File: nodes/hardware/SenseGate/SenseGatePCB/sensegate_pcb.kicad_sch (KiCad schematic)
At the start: 25 parts, among them J1 Conn_01x02_Pin, J10 Conn_01x02_Pin, J11 Conn_01x02_Pin, J2 Conn_01x02_Socket, J3 Conn_01x02_Socket, J4 Conn_01x24_Pin, J5 Conn_01x04_Socket, J6 Conn_01x04_Socket, J7 Conn_01x04_Socket, J8 Conn_01x04_Socket, J9 Conn_01x02_Socket, Q4 SS8050, SW1 SW_Reed, SW2 SW_Reed, SW3 SW_Reed, SW5 SW_DPDT_x2, U1 DD05CVSA

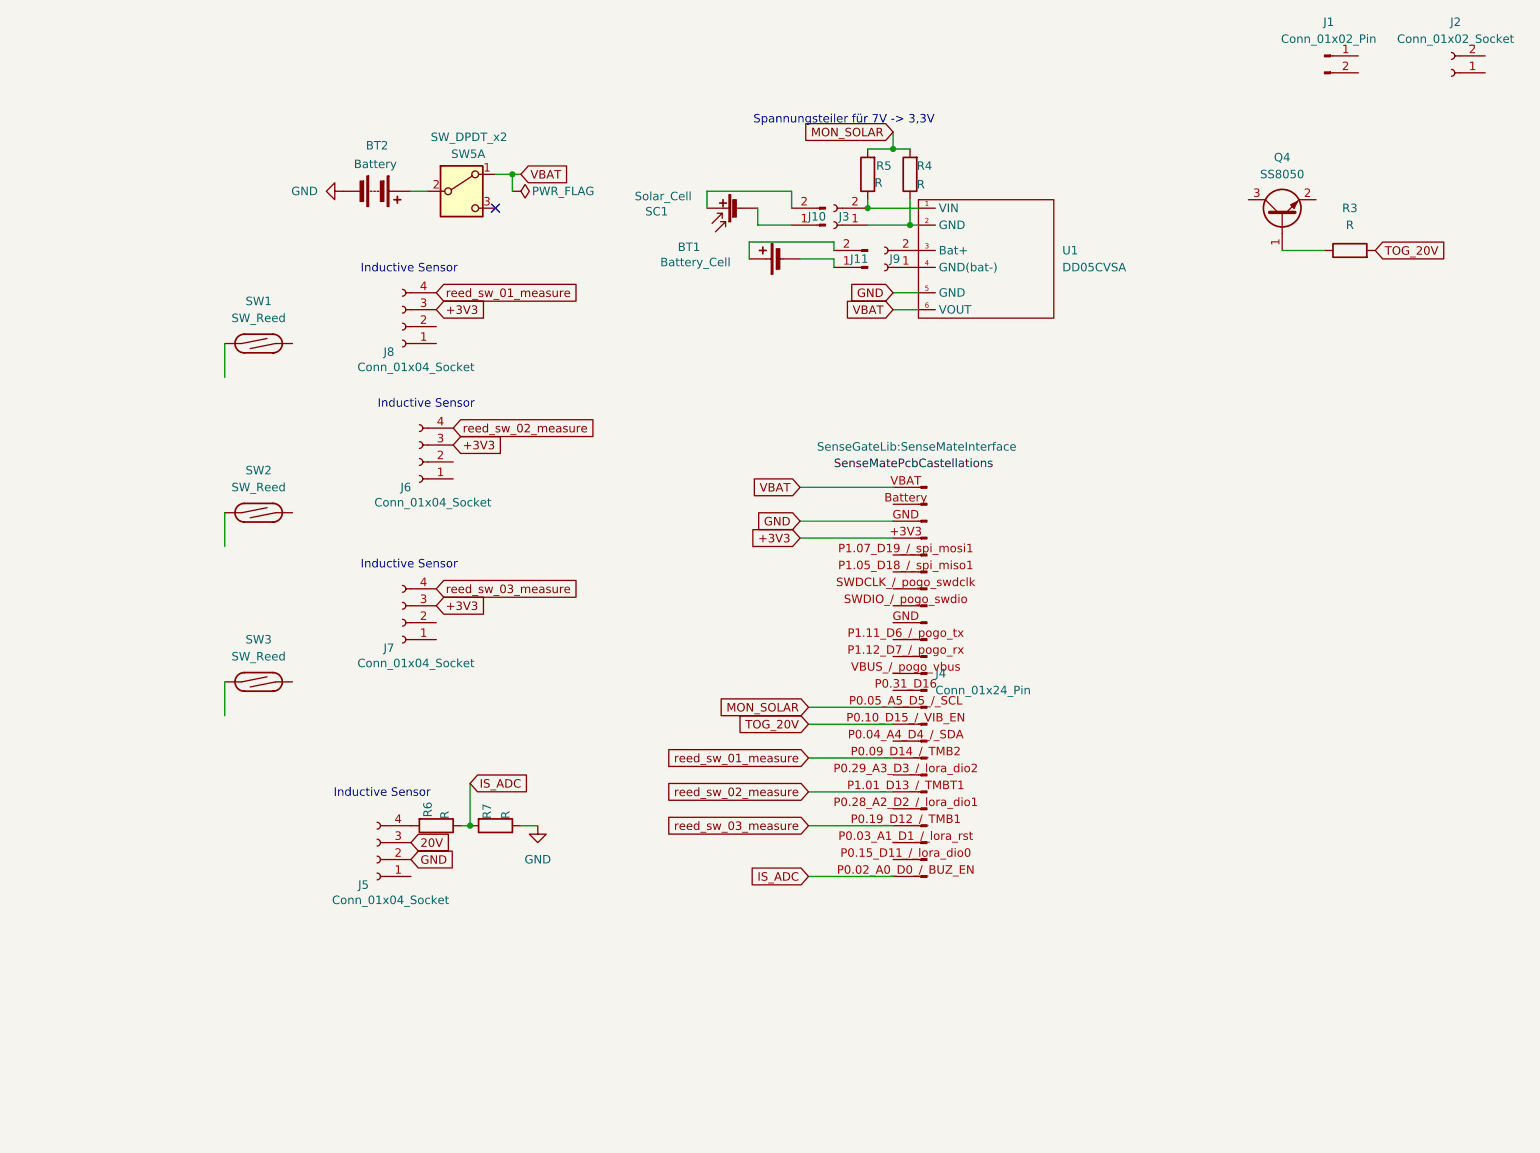
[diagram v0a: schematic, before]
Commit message: schematic done
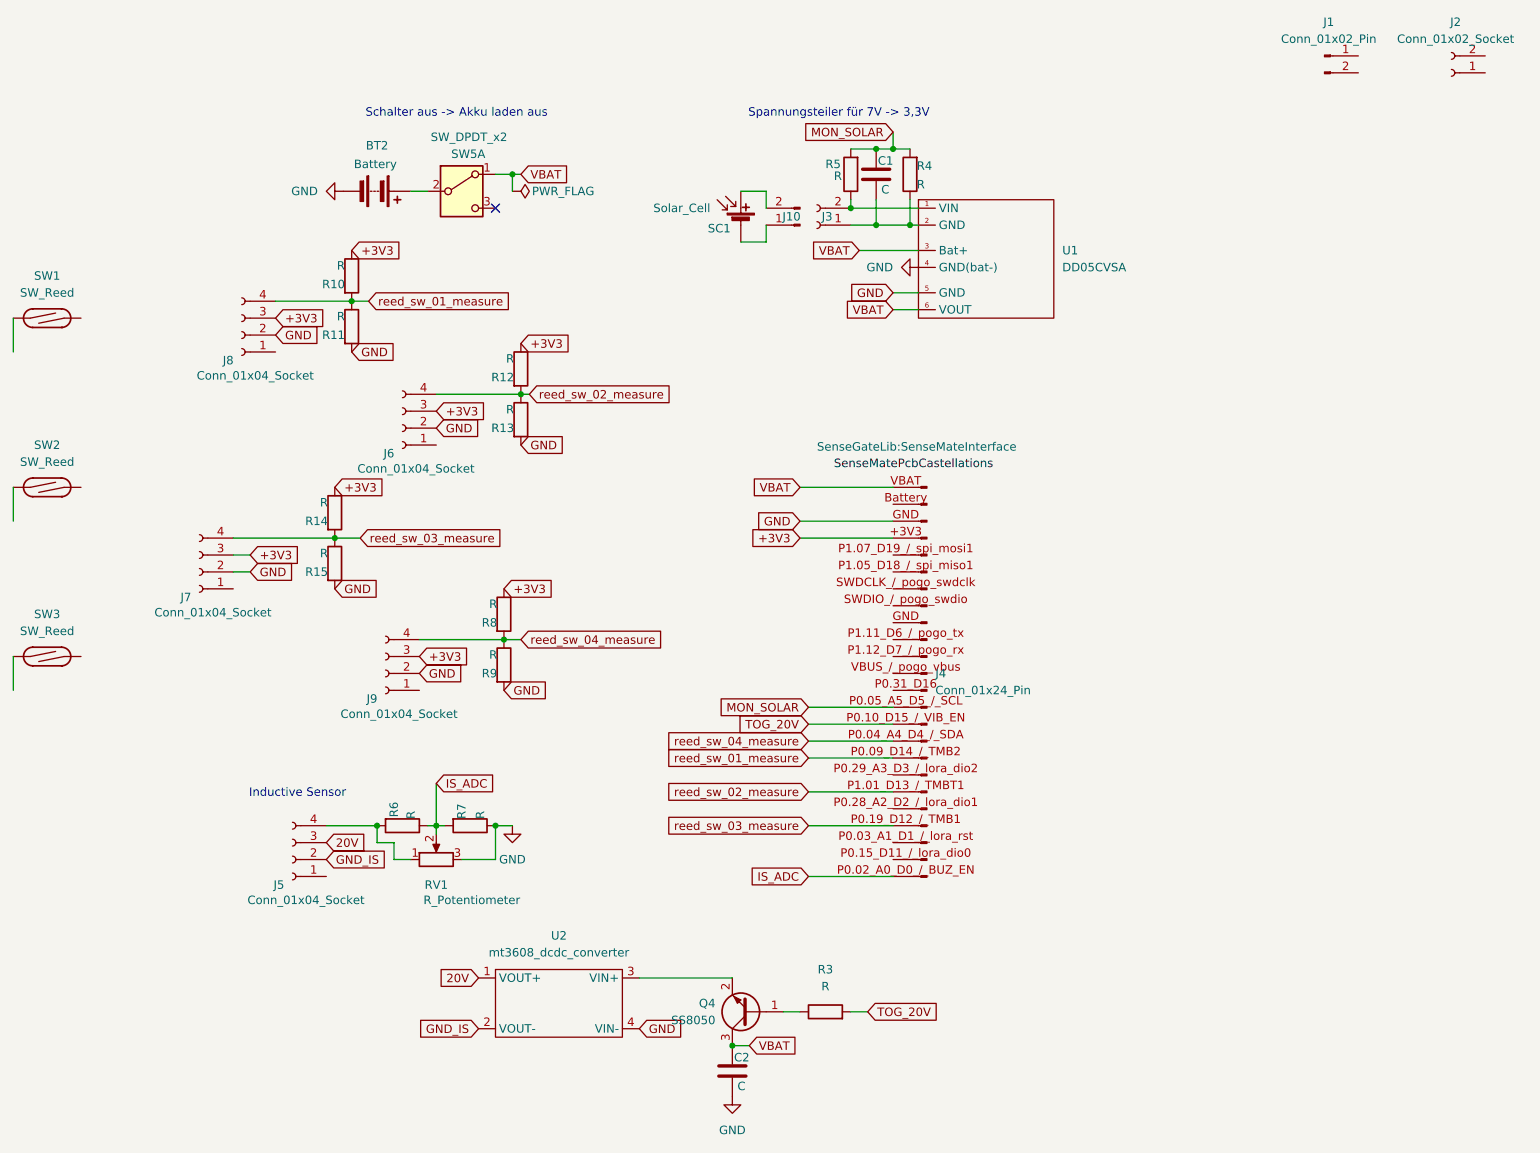
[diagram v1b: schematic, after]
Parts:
- removed BT1: Battery_Cell, symbol Device:Battery_Cell
- removed J11: Conn_01x02_Pin, symbol Connector:Conn_01x02_Pin
- removed J9: Conn_01x02_Socket, symbol Connector:Conn_01x02_Socket
- added C1, C2: C, symbol Device:C
- added J9: Conn_01x04_Socket, Connector_JST:JST_PH_B4B-PH-K_1x04_P2.00mm_Vertical, symbol Connector:Conn_01x04_Socket
- added R10, R11, R12, R13, R14, R15, R8, R9: R, Resistor_SMD:R_0805_2012Metric, symbol Device:R
- added RV1: R_Potentiometer, symbol Device:R_Potentiometer
- added U2: mt3608_dcdc_converter, custom_dcdc_converters:MT3608_solarbotics, symbol custom_symbols:mt3608_dcdc_converter
- J3: footprint (none) -> Connector_JST:JST_PH_B2B-PH-K_1x02_P2.00mm_Vertical
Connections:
- net +3V3: now also J9.3 (Pin_3), R10.1, R12.1, R14.1, R8.1
- net 20V: now also U2.1 (VOUT+)
- net GND: now also J6.2 (Pin_2), J7.2 (Pin_2), J8.2 (Pin_2), U1.4 (GND(bat-)), C2.2, J9.2 (Pin_2), R11.2, R13.2, R15.2, R9.2, RV1.3, U2.4 (VIN-); no longer J5.2 (Pin_2)
- net IS_ADC: now also RV1.2
- net MON_SOLAR: now also C1.1
- net VBAT: now also Q4.3 (C), U1.3 (Bat+), C2.1
- net reed_sw_01_measure: now also R10.2, R11.1
- net reed_sw_02_measure: now also R12.2, R13.1
- net reed_sw_03_measure: now also R14.2, R15.1
- net at Q4.2 (E): now also U2.3 (VIN+)
- net at J5.4 (Pin_4), R6.2: now also RV1.1
- net at J3.1 (Pin_1), R4.1, U1.2 (GND): now also C1.2
- net reed_sw_04_measure: now reaches J4.P0.04_A4_D4_/_SDA (9)
- net reed_sw_04_measure: now also J9.4 (Pin_4), R8.2, R9.1
- new net GND_IS: J5.2 (Pin_2), U2.2 (VOUT-)
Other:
- note added: "Schalter aus -> Akku laden aus"
- moved on the sheet: J10, J3, J5, J6, J7, J8, Q4, R3, R5, R6, R7, SC1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
